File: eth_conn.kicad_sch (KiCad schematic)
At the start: 30 parts, among them J1 RJ45

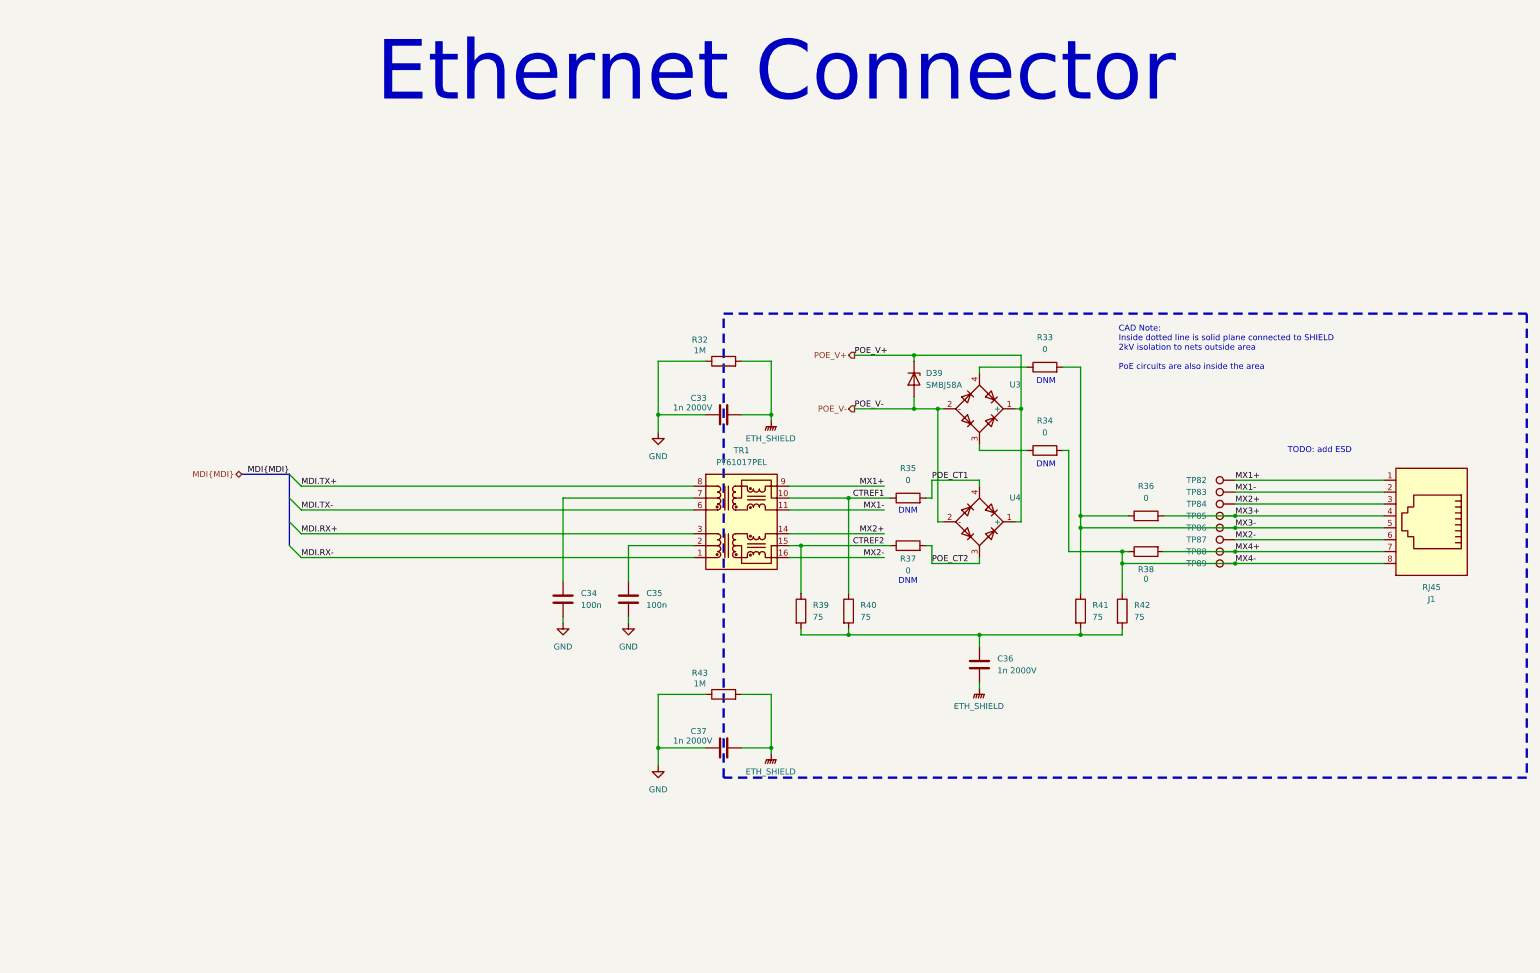
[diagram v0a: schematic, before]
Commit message: many stuffs
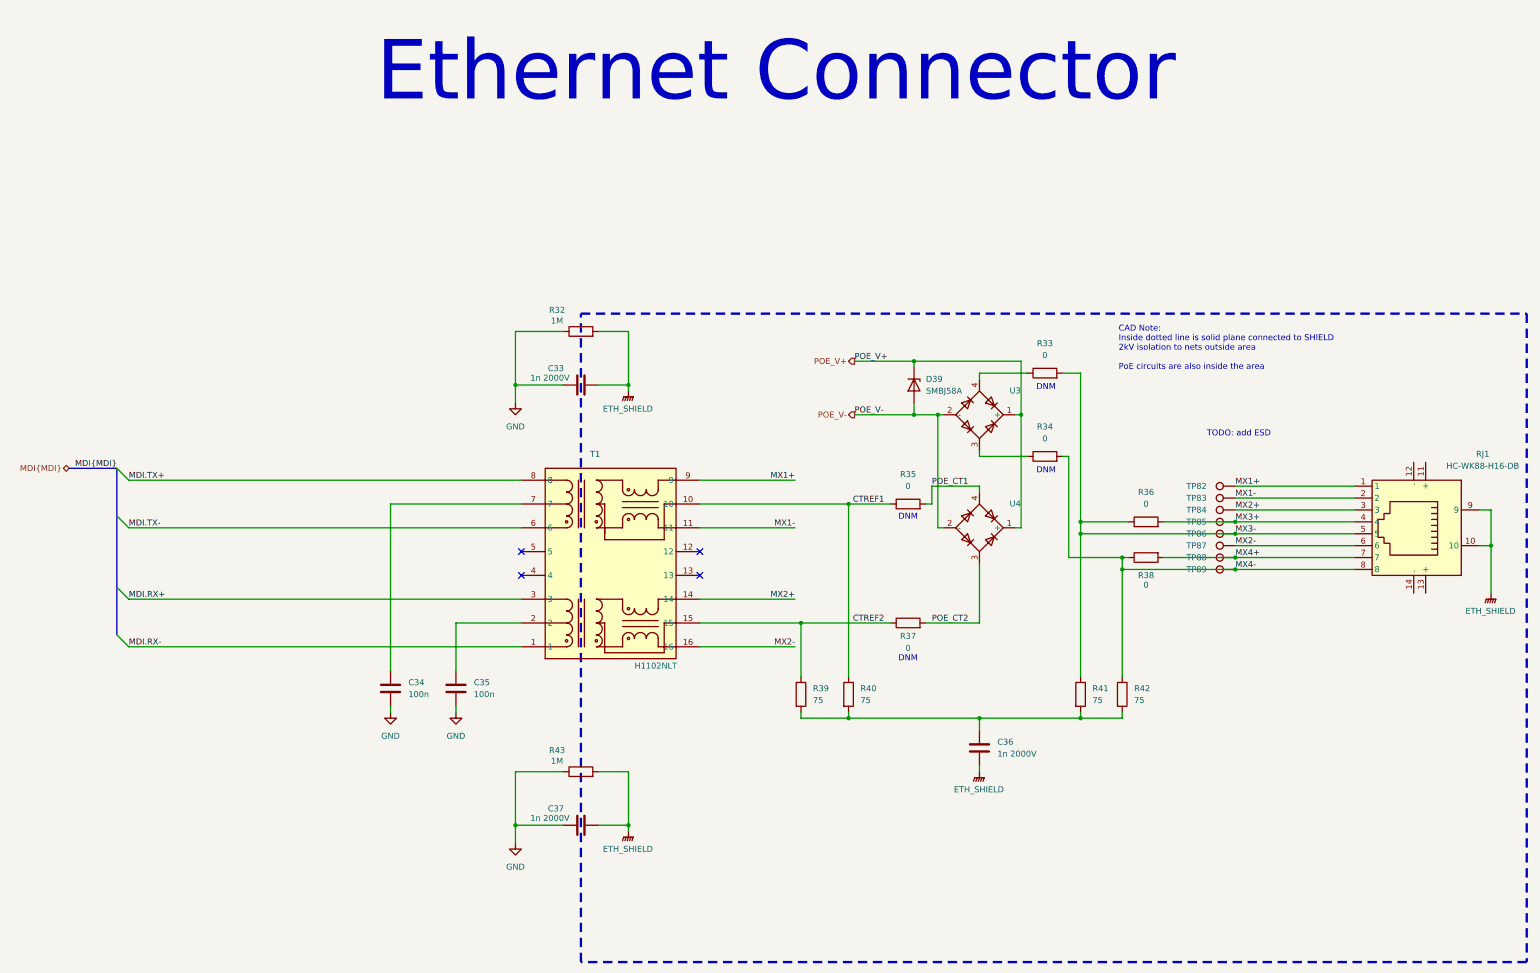
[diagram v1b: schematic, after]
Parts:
- removed J1: RJ45, Connector_RJ:RJ45_Amphenol_54602-x08_Horizontal, symbol Connector:RJ45
- removed TR1: PT61017PEL, Transformer_SMD:Transformer_Ethernet_Bourns_PT61017PEL, symbol Transformer:PT61017PEL
- added RJ1: HC-WK88-H16-DB, C7501824:RJ45-TH_HC-WK88-H16-DB, symbol C7501824:HC-WK88-H16-DB
- added T1: H1102NLT, C18584:XFMR-SMD_H1102NLT, symbol C18584:H1102NLT
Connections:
- net CTREF1: now also T1.10
- net CTREF2: now also T1.15
- net ETH_SHIELD: now also RJ1.10, RJ1.9
- net MDI.RX+: now also T1.3
- net MDI.RX-: now also T1.1
- net MDI.TX+: now also T1.8
- net MDI.TX-: now also T1.6
- net MX1+: now also RJ1.1, T1.9
- net MX1-: now also RJ1.2, T1.11
- net MX2+: now also RJ1.3, T1.14
- net MX2-: now also RJ1.6, T1.16
- net MX3+: now also RJ1.4
- net MX3-: now also RJ1.5
- net MX4+: now also RJ1.7
- net MX4-: now also RJ1.8
- net at C35.1: now also T1.2
- net at C34.1: now also T1.7
- no-connect marks 0 -> 4
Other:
- moved on the sheet: C33, C36, C37, D39, R32, R33, R34, R35, R36, R37, R38, R39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
